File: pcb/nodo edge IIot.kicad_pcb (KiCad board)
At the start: 2 copper layers, 100 x 70 mm, 11 parts, among them J1 ESP32_DEVKIT_38P, J2 PZEM_004T, J3 DC_IN

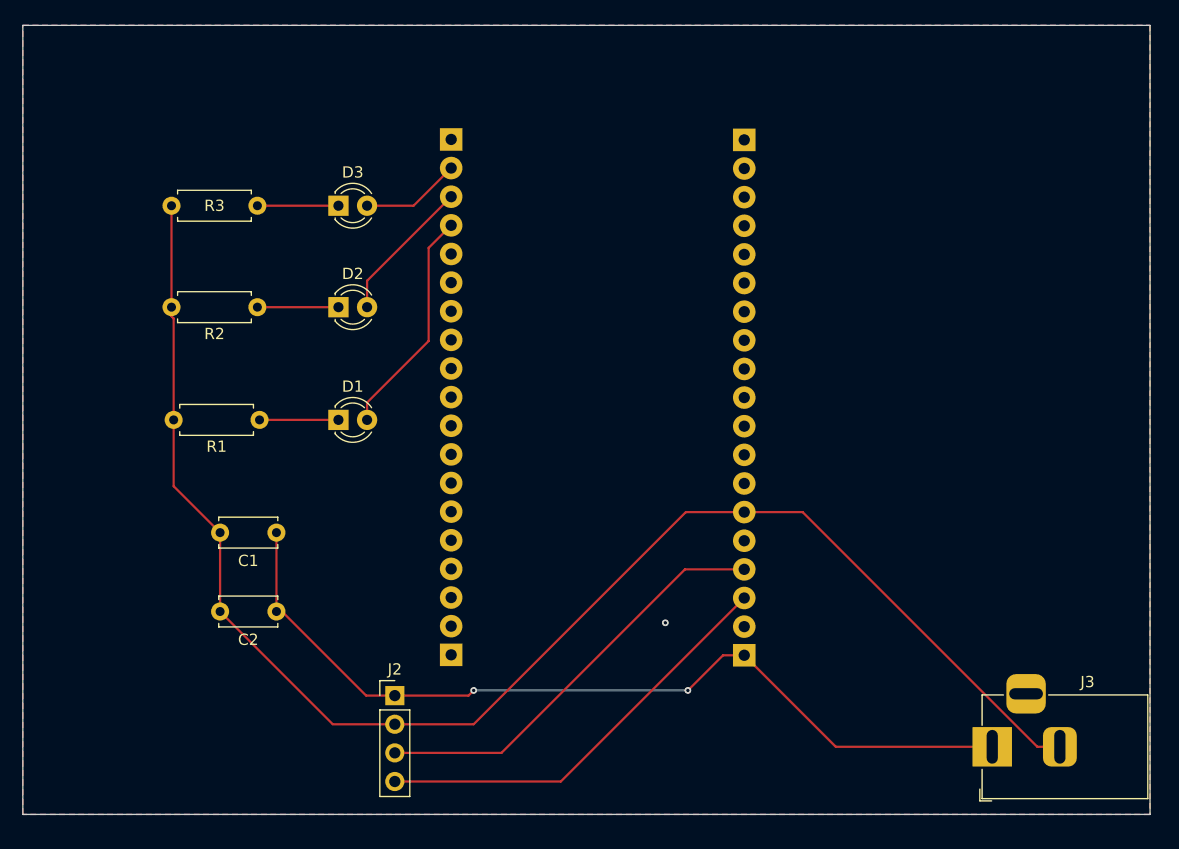
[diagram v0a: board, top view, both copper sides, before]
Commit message: Update PCB design
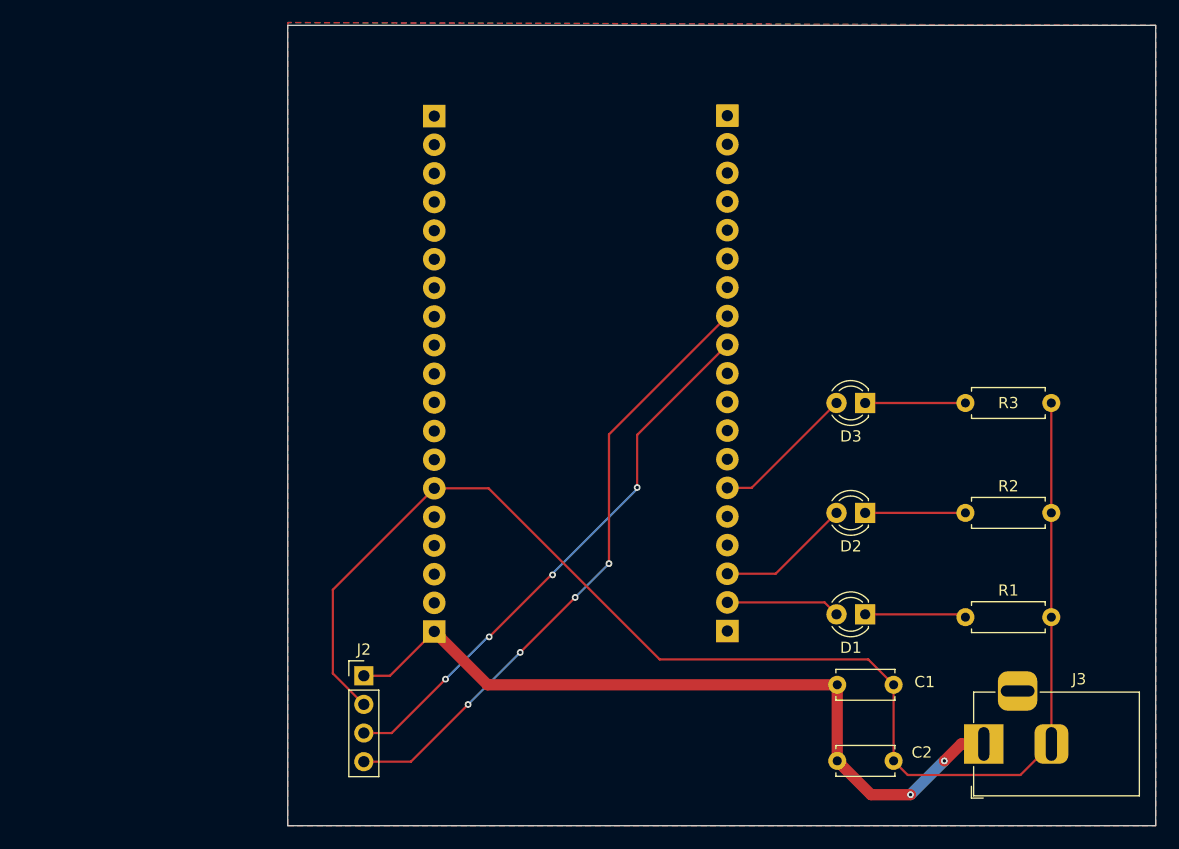
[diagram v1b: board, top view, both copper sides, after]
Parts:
- removed J1: ESP32_DEVKIT_38P, Esp 38 pin:ESP32-38pin
- added ESP32_38P1: ~, Esp 38 pin:ESP32-38pin, B.Cu at (116.0, 59.9)
- moved R2 65.4 mm to (151.6, 72.2), turned to 0 degrees
- moved R3 65.2 mm to (151.6, 62.5), turned to 0 degrees
- moved R1 65.0 mm to (151.6, 81.5), turned to 0 degrees
- moved C1 51.5 mm to (140.2, 87.5), turned to 0 degrees
- moved C2 51.5 mm to (140.2, 94.2), turned to 0 degrees
- moved D2 50.2 mm to (142.7, 72.2), turned to 180 degrees
- moved D3 49.9 mm to (142.7, 62.5), turned to 180 degrees
- moved D1 49.8 mm to (142.7, 81.2), turned to 180 degrees
- moved J2 3.26 mm to (98.2, 86.7)
- moved J3 0.79 mm to (153.2, 92.8)
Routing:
- net /RX_PZEM: track 37.7 -> 55.3 mm, vias 0 -> 4
- net /TX_PZEM: track 37.7 -> 49.4 mm, vias 0 -> 4
- net /GPIO23: track 20.4 -> 10.1 mm
- net /VIN: track 78.4 -> 68.7 mm
- net GND: track 132.8 -> 124.7 mm, vias 1 -> 0
- net /GPIO21: track 8.84 -> 12.9 mm
- net Net-(D1-K): track 7.00 -> 9.35 mm
- net Net-(D3-K): track 7.19 -> 8.90 mm
- net Net-(D2-K): track 7.19 -> 8.90 mm
- net /GPIO22: track 12.9 -> 11.9 mm
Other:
- board size 100 x 70 mm -> 77 x 71 mm
